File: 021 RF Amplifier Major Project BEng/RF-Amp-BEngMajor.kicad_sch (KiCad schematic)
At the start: 32 parts, among them SW1 SW_SPDT, U1 THS4302RGTT

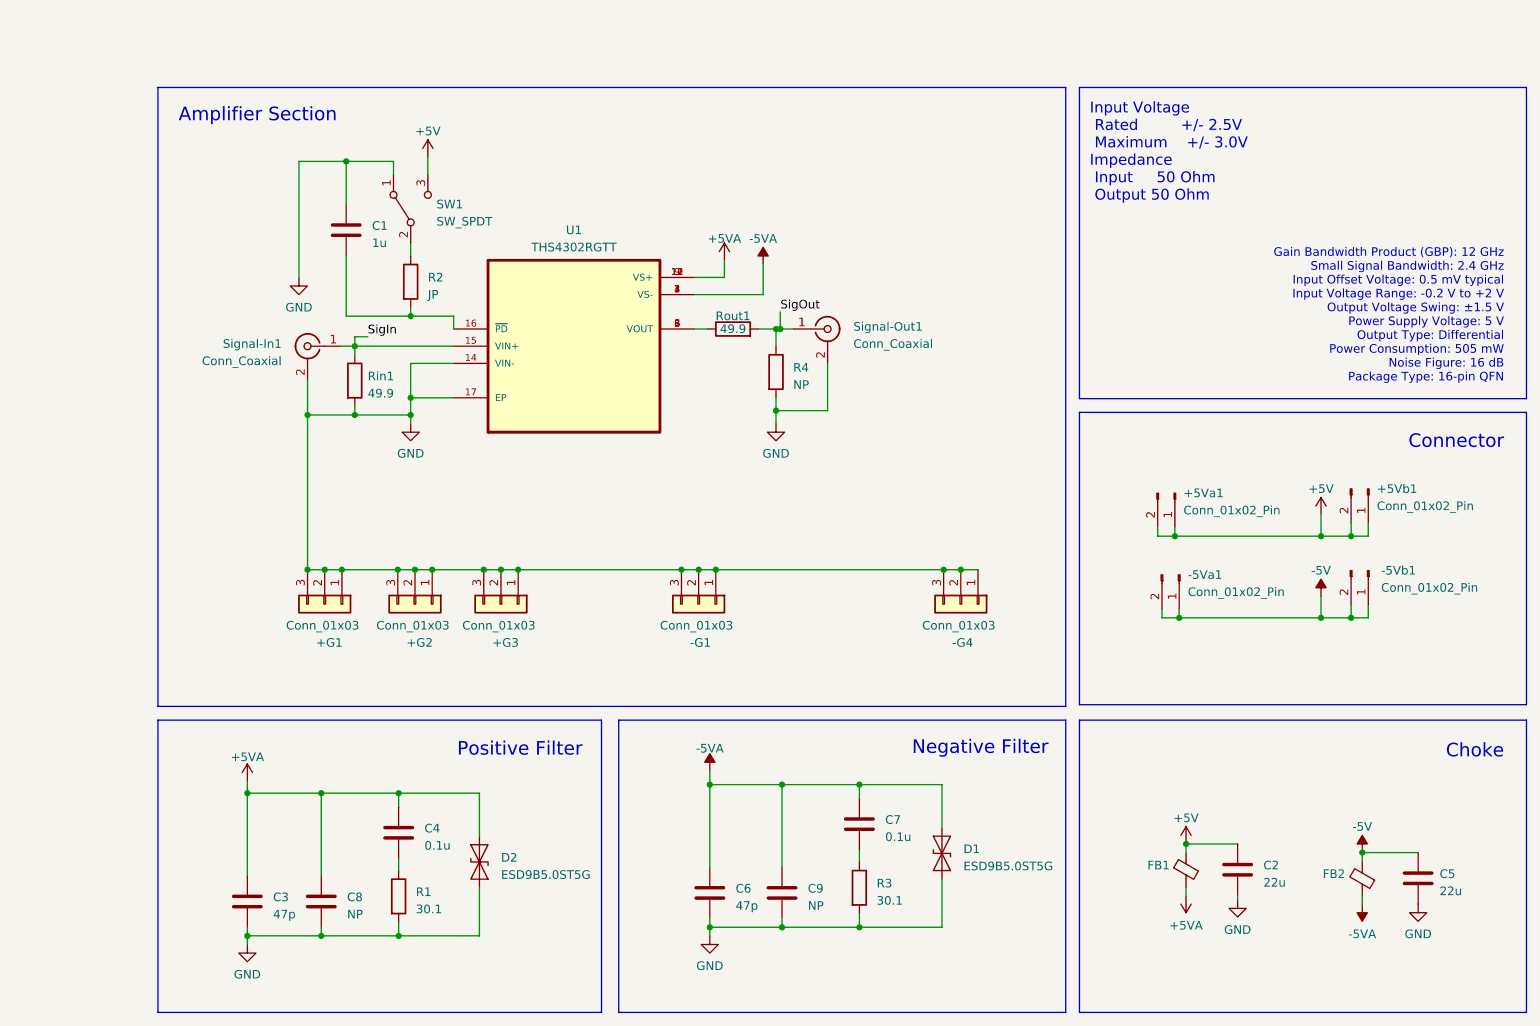
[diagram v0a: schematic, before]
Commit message: Comments Modified
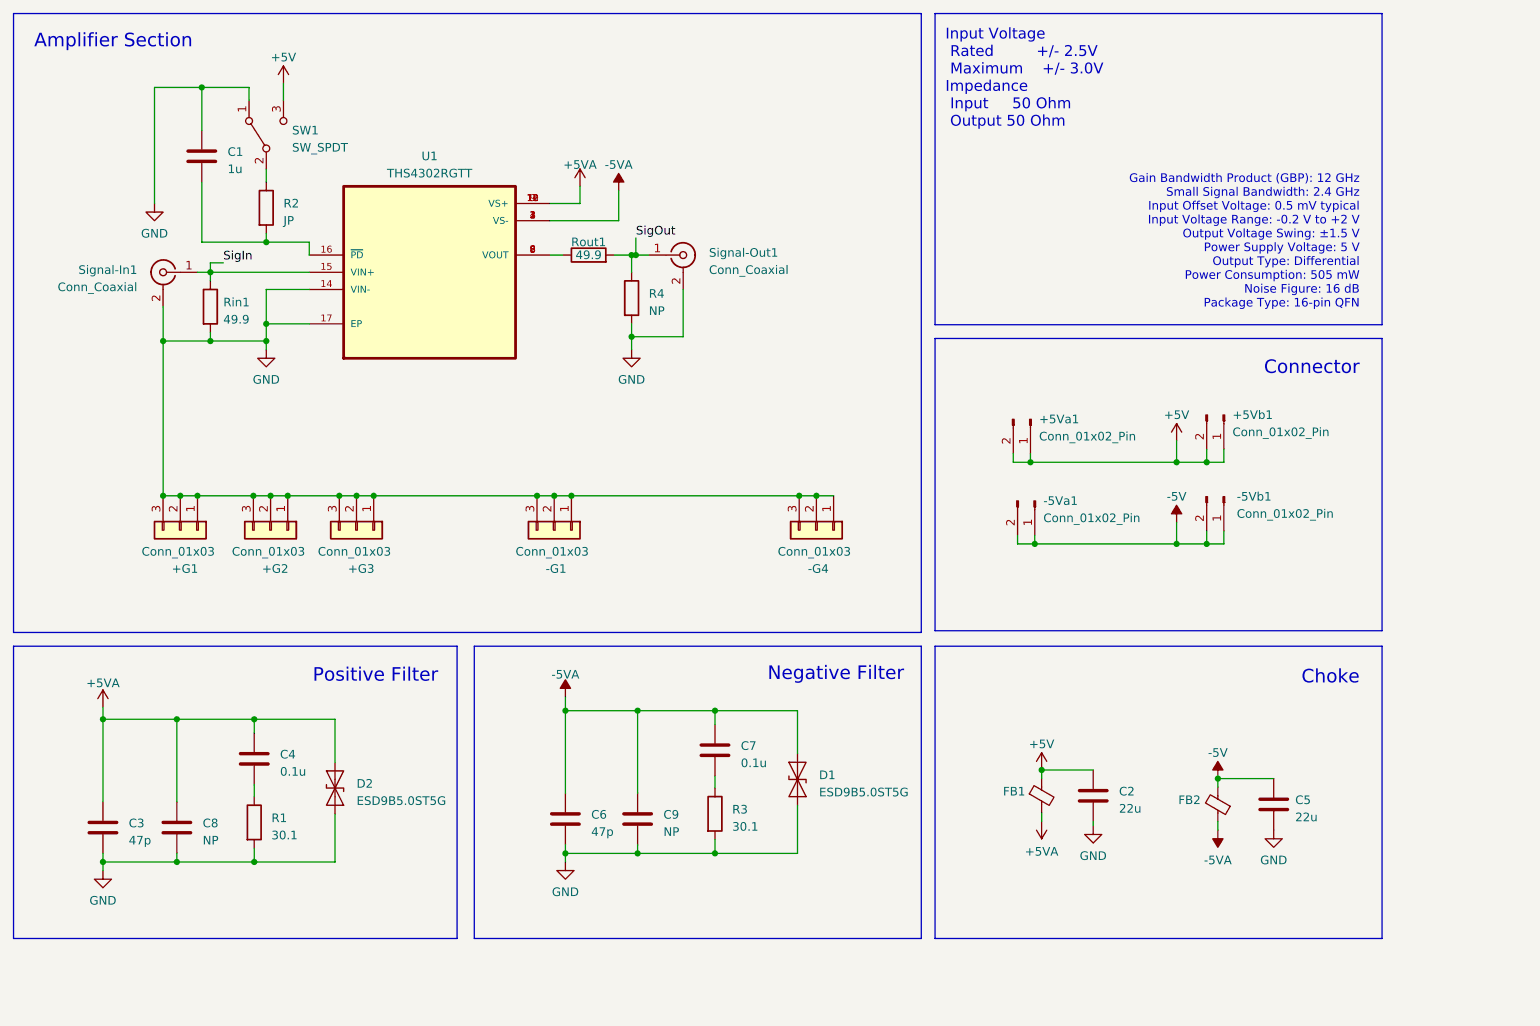
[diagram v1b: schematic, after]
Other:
- moved on the sheet: +5Va1, +5Vb1, +G1, +G2, +G3, -5Va1, -5Vb1, -G1, -G4, C1, C2, C3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
